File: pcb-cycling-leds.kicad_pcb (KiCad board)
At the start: 2 copper layers, 206 x 9.7 mm, 30 parts, among them J1 Power, J2 LED, J3 Sensor, U1 SC4011

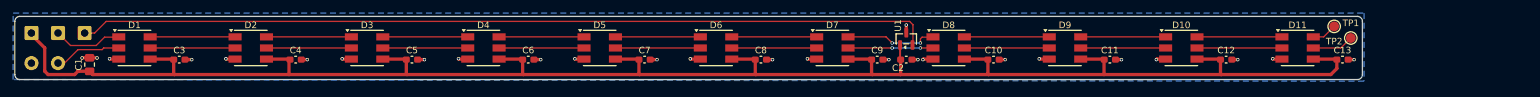
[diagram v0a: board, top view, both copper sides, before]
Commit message: Finish routing
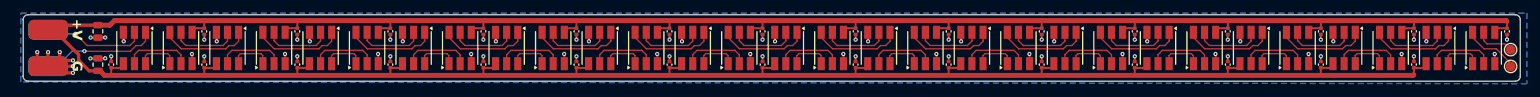
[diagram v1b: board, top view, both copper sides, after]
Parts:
- removed U1: SC4011, Package_TO_SOT_SMD:SOT-23
- added C14: 0.1uF, Capacitor_SMD:C_0402_1005Metric, F.Cu at (125.5, 58.2)
- added C15: 0.1uF, Capacitor_SMD:C_0402_1005Metric, F.Cu at (139.7, 53.1)
- added C16: 0.1uF, Capacitor_SMD:C_0402_1005Metric, F.Cu at (139.7, 58.2)
- added C17: 0.1uF, Capacitor_SMD:C_0402_1005Metric, F.Cu at (153.9, 53.1)
- added C18: 0.1uF, Capacitor_SMD:C_0402_1005Metric, F.Cu at (153.9, 58.2)
- added C19: 0.1uF, Capacitor_SMD:C_0402_1005Metric, F.Cu at (168.1, 53.1)
- added C20: 0.1uF, Capacitor_SMD:C_0402_1005Metric, F.Cu at (168.1, 58.2)
- added C21: 0.1uF, Capacitor_SMD:C_0402_1005Metric, F.Cu at (182.4, 53.1)
- added C22: 0.1uF, Capacitor_SMD:C_0402_1005Metric, F.Cu at (182.4, 58.2)
- added C23: 0.1uF, Capacitor_SMD:C_0402_1005Metric, F.Cu at (196.6, 53.1)
- added C24: 0.1uF, Capacitor_SMD:C_0402_1005Metric, F.Cu at (196.6, 58.2)
- added C25: 0.1uF, Capacitor_SMD:C_0402_1005Metric, F.Cu at (210.8, 53.1)
- added C26: 0.1uF, Capacitor_SMD:C_0402_1005Metric, F.Cu at (210.8, 58.2)
- added C27: 0.1uF, Capacitor_SMD:C_0402_1005Metric, F.Cu at (225.0, 53.1)
- added C28: 0.1uF, Capacitor_SMD:C_0402_1005Metric, F.Cu at (225.0, 58.2)
- added C29: 0.1uF, Capacitor_SMD:C_0402_1005Metric, F.Cu at (239.3, 53.1)
- added C30: 0.1uF, Capacitor_SMD:C_0402_1005Metric, F.Cu at (239.3, 58.2)
- added C31: 0.1uF, Capacitor_SMD:C_0402_1005Metric, F.Cu at (253.5, 53.1)
- added C32: 10uF, Capacitor_SMD:C_0805_2012Metric, F.Cu at (38.1, 53.1)
- added D12: APA102, LED_SMD:LED_RGB_5050-6, F.Cu at (121.9, 55.6)
- added D13: APA102, LED_SMD:LED_RGB_5050-6, F.Cu at (129.0, 55.6)
- added D14: APA102, LED_SMD:LED_RGB_5050-6, F.Cu at (136.1, 55.6)
- added D15: APA102, LED_SMD:LED_RGB_5050-6, F.Cu at (143.3, 55.6)
- added D16: APA102, LED_SMD:LED_RGB_5050-6, F.Cu at (150.4, 55.6)
- added D17: APA102, LED_SMD:LED_RGB_5050-6, F.Cu at (157.5, 55.6)
- added D18: APA102, LED_SMD:LED_RGB_5050-6, F.Cu at (164.6, 55.6)
- added D19: APA102, LED_SMD:LED_RGB_5050-6, F.Cu at (171.7, 55.6)
- added D20: APA102, LED_SMD:LED_RGB_5050-6, F.Cu at (178.8, 55.6)
- added D21: APA102, LED_SMD:LED_RGB_5050-6, F.Cu at (185.9, 55.6)
- added D22: APA102, LED_SMD:LED_RGB_5050-6, F.Cu at (193.0, 55.6)
- added D23: APA102, LED_SMD:LED_RGB_5050-6, F.Cu at (200.2, 55.6)
- added D24: APA102, LED_SMD:LED_RGB_5050-6, F.Cu at (207.3, 55.6)
- added D25: APA102, LED_SMD:LED_RGB_5050-6, F.Cu at (214.4, 55.6)
- added D26: APA102, LED_SMD:LED_RGB_5050-6, F.Cu at (221.5, 55.6)
- added D27: APA102, LED_SMD:LED_RGB_5050-6, F.Cu at (228.6, 55.6)
- added D28: APA102, LED_SMD:LED_RGB_5050-6, F.Cu at (235.7, 55.6)
- added D29: APA102, LED_SMD:LED_RGB_5050-6, F.Cu at (242.8, 55.6)
- added D30: APA102, LED_SMD:LED_RGB_5050-6, F.Cu at (249.9, 55.6)
- added J4: G, Connector_Wire:SolderWirePad_1x01_SMD_3x6mm, F.Cu at (30.5, 58.4)
- C1: footprint Capacitor_SMD:C_0805_2012Metric_Pad1.18x1.45mm_HandSolder -> Capacitor_SMD:C_0805_2012Metric
- C10, C11, C12, C13, C2, C3, C4, C5, C6, C7, C8, C9: footprint Capacitor_SMD:C_0603_1608Metric_Pad1.08x0.95mm_HandSolder -> Capacitor_SMD:C_0402_1005Metric
- J1: value Power -> V; footprint Connector_Wire:SolderWire-0.5sqmm_1x02_P4.6mm_D0.9mm_OD2.1mm -> Connector_Wire:SolderWirePad_1x01_SMD_3x6mm
- J2: value LED -> D; footprint Connector_Wire:SolderWire-0.5sqmm_1x02_P4.6mm_D0.9mm_OD2.1mm -> Connector_Wire:SolderWirePad_1x01_SMD_3x6mm; moved to B.Cu
- J3: value Sensor -> C; footprint Connector_Wire:SolderWire-0.5sqmm_1x01_D0.9mm_OD2.1mm -> Connector_Wire:SolderWirePad_1x01_SMD_3x6mm; moved to B.Cu
- moved C2 121.5 mm to (40.1, 58.2), turned to 90 degrees
- moved D11 106.7 mm to (114.8, 55.6), turned to -90 degrees
- moved C13 103.0 mm to (125.5, 53.1), turned to -90 degrees
- moved C12 99.3 mm to (111.3, 58.2), turned to 90 degrees
- moved D10 96.0 mm to (107.7, 55.6), turned to 90 degrees
- moved D9 85.3 mm to (100.6, 55.6), turned to -90 degrees
- moved C11 81.6 mm to (111.3, 53.1), turned to -90 degrees
- moved C10 78.0 mm to (97.0, 58.2), turned to 90 degrees
- moved D8 74.7 mm to (93.5, 55.6), turned to 90 degrees
- moved D7 64.0 mm to (86.4, 55.6), turned to -90 degrees
- moved C9 60.4 mm to (97.0, 53.1), turned to -90 degrees
- moved C8 56.6 mm to (82.8, 58.2), turned to 90 degrees
- moved D6 53.3 mm to (79.2, 55.6), turned to 90 degrees
- moved D5 42.7 mm to (72.1, 55.6), turned to -90 degrees
- moved C7 39.1 mm to (82.8, 53.1), turned to -90 degrees
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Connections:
- J3 pad 1: SENSOR -> LED_CLK
- TP1 pad 1: Net-(D11-DO) -> Net-(D30-DO)
- TP2 pad 1: Net-(D11-CO) -> Net-(D30-CO)
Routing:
- net VCC: track 274.3 -> 542.0 mm
- net SENSOR: track 130.7 -> 0.00 mm
- net GND: track 31.1 -> 93.0 mm, vias 26 -> 70
- net Net-(D26-DO): track 0.00 -> 13.9 mm
- net Net-(D24-DO): track 0.00 -> 13.9 mm
- net Net-(D14-DO): track 0.00 -> 13.9 mm
- net Net-(D28-DO): track 0.00 -> 13.9 mm
- net Net-(D18-DO): track 0.00 -> 13.9 mm
- net Net-(D16-DO): track 0.00 -> 13.9 mm
- net Net-(D12-DO): track 0.00 -> 13.9 mm
- net Net-(D22-DO): track 0.00 -> 13.9 mm
- net Net-(D20-DO): track 0.00 -> 13.9 mm
- net Net-(D23-CO): track 0.00 -> 10.4 mm
- net Net-(D17-CO): track 0.00 -> 10.4 mm
- net Net-(D29-CO): track 0.00 -> 10.4 mm
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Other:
- board size 206 x 9.7 mm -> 228.9 x 10.2 mm
- board text added: "+V"
- board text added: "C"
- board text added: "C D"
- board text added: "D"
- board text added: "G"
- board text added: "JLCJLCJLCJLC"
- board text added: "REV 1"
